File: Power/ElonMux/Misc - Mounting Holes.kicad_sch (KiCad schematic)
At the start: 12 parts

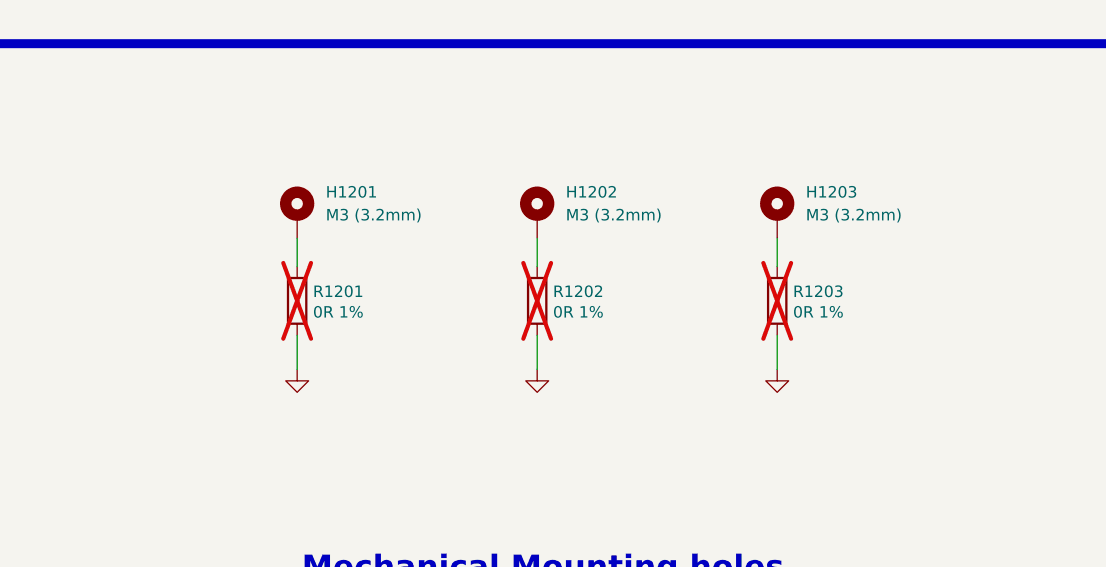
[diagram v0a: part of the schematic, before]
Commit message: Implemented more fede recommandations
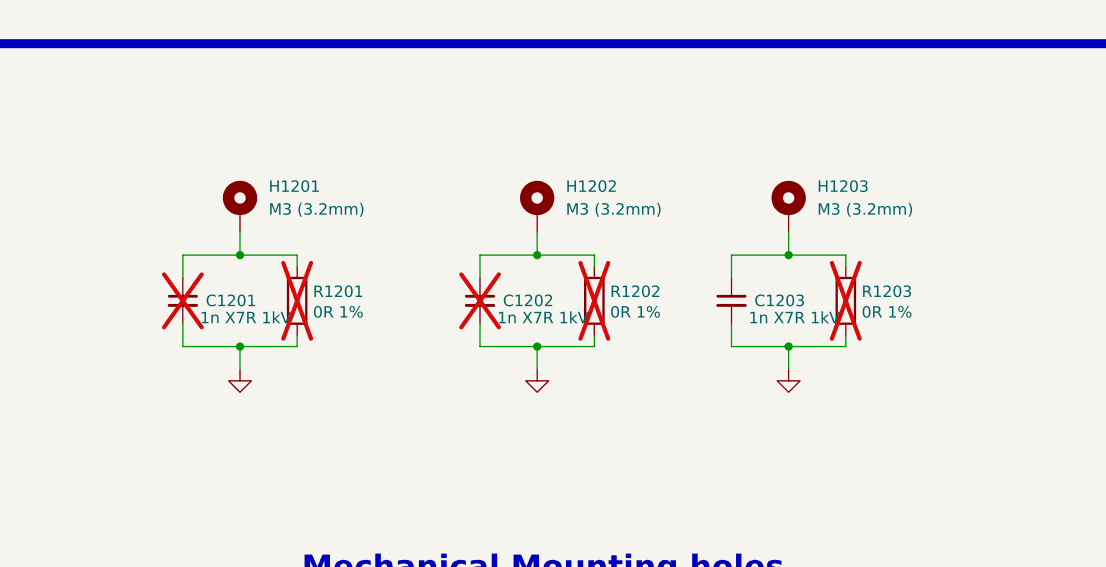
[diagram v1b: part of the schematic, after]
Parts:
- added C1201, C1202, C1203: 1n X7R 1kV, Capacitor_SMD:C_0603_1608Metric, symbol Device:C_Small
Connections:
- net GND: now also C1201.2, C1202.2, C1203.2
- net at H1203.1, R1203.1: now also C1203.1
- net at H1202.1, R1202.1: now also C1202.1
- net at H1201.1, R1201.1: now also C1201.1
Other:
- moved on the sheet: H1201
